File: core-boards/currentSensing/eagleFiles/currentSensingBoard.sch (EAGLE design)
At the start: 22 parts, among them Q1 16MHz, X1 3-PIN_2MM-H, X2 2-PIN_2MM-H, X3 4-PIN_2MM-H

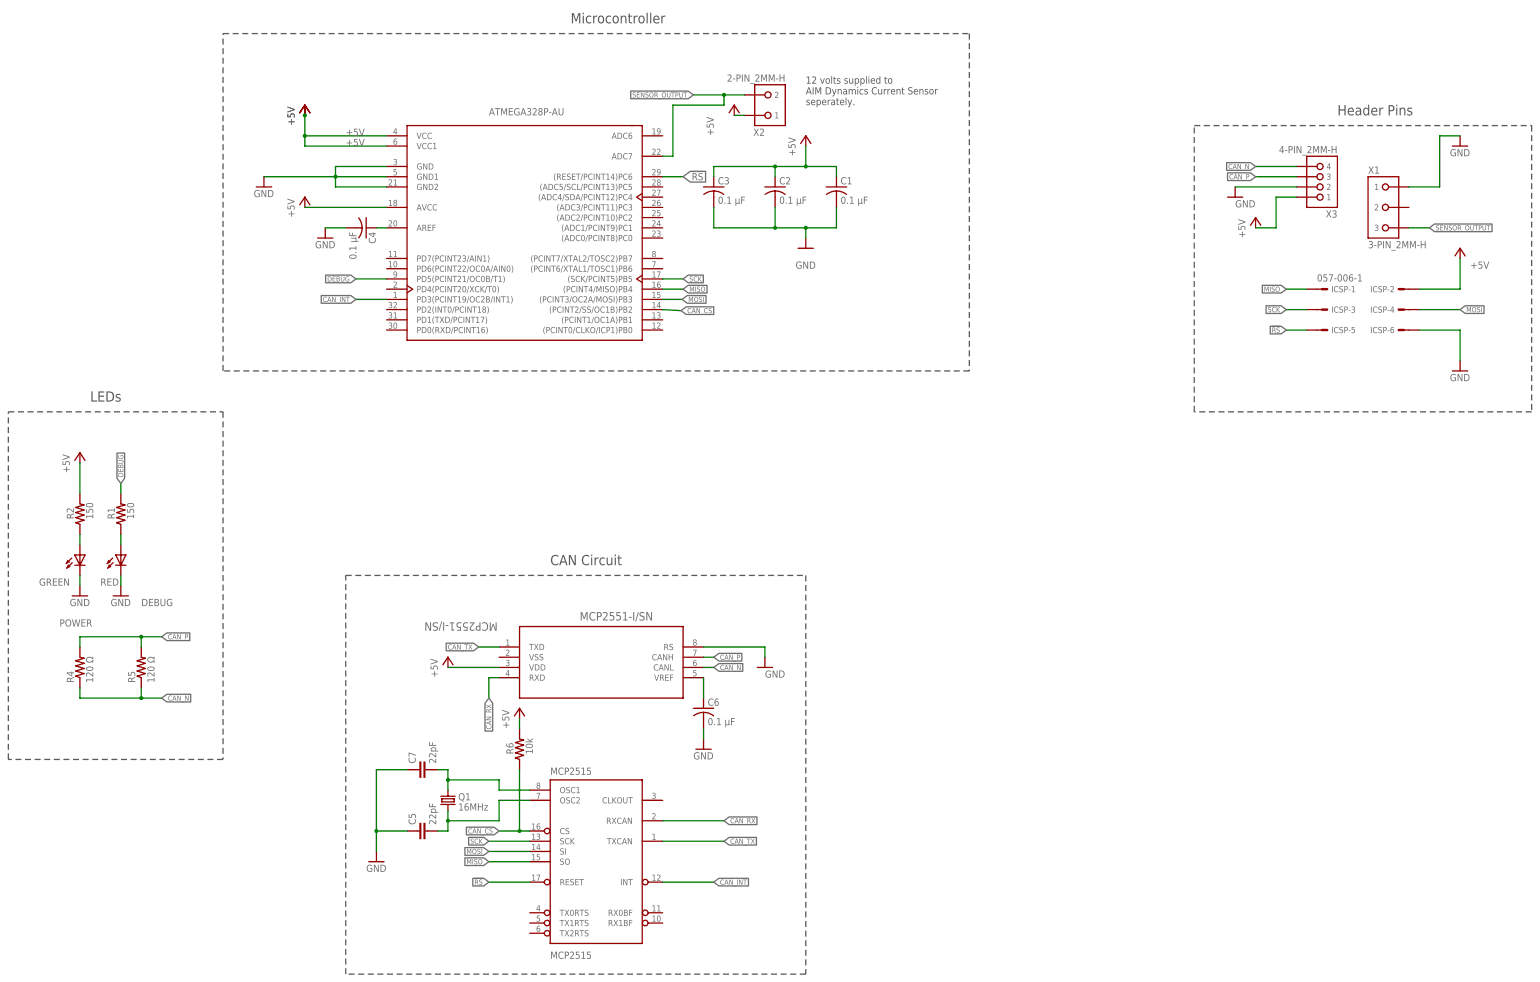
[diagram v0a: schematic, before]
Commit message: Changes to Board Complete
-Most recent round of commentes taken account of
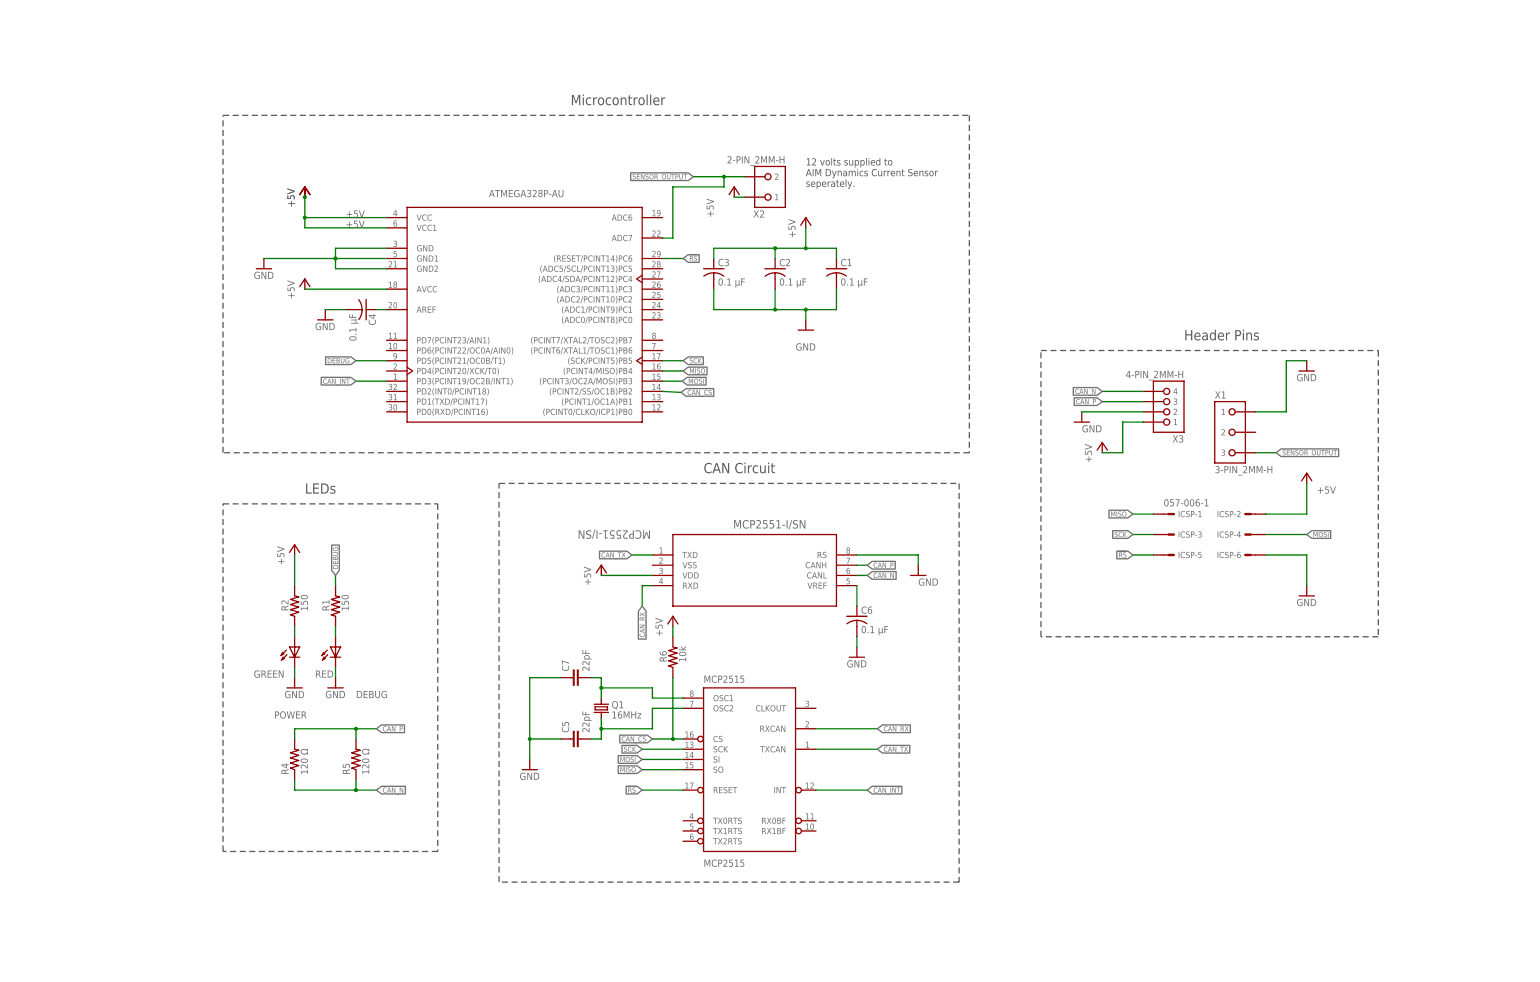
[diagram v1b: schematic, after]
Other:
- moved on the sheet: C1, C2, C3, C4, C5, C6, C7, DEBUG, ICSP-1, ICSP-2, ICSP-3, ICSP-4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
